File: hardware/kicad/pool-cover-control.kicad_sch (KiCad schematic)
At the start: 70 parts, among them J1 Power_Supply _Conn, J2 Motor_Conn, J3 Key_Switch_Conn, J4 Limit_Switch_Conn, J5 SWD_Conn, Q1 DMP4015SK3Q-13, U1 STM32G031K8Tx, U2 ULN2003A, U3 LMR14206, U4 PC817, U5 PC817, U6 PC817, U7 PC817

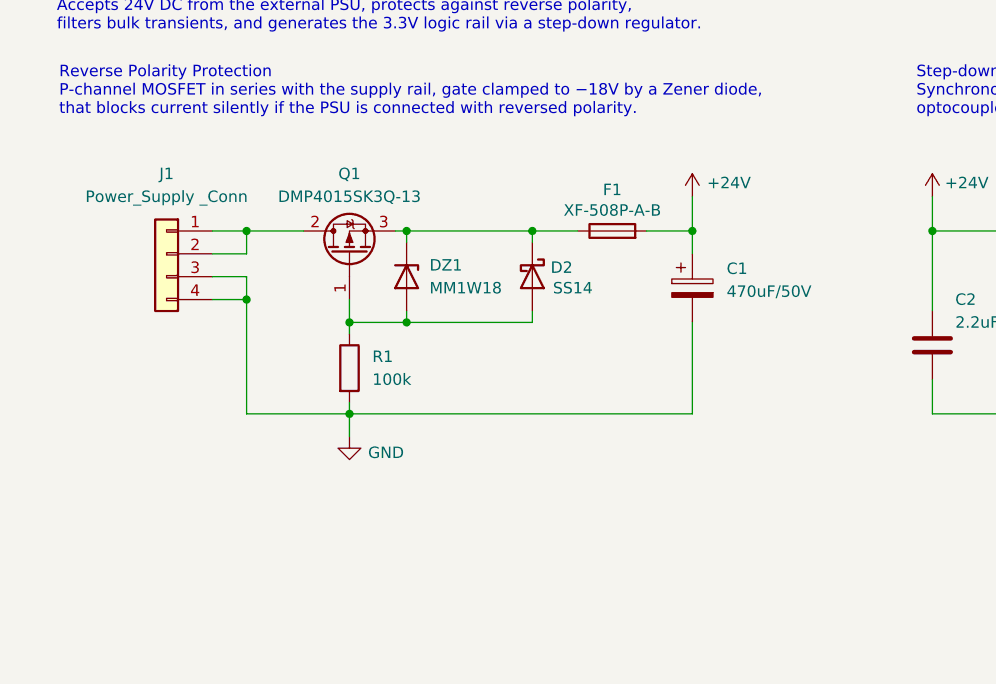
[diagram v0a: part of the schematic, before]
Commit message: feat(hardware): implement pcb layout
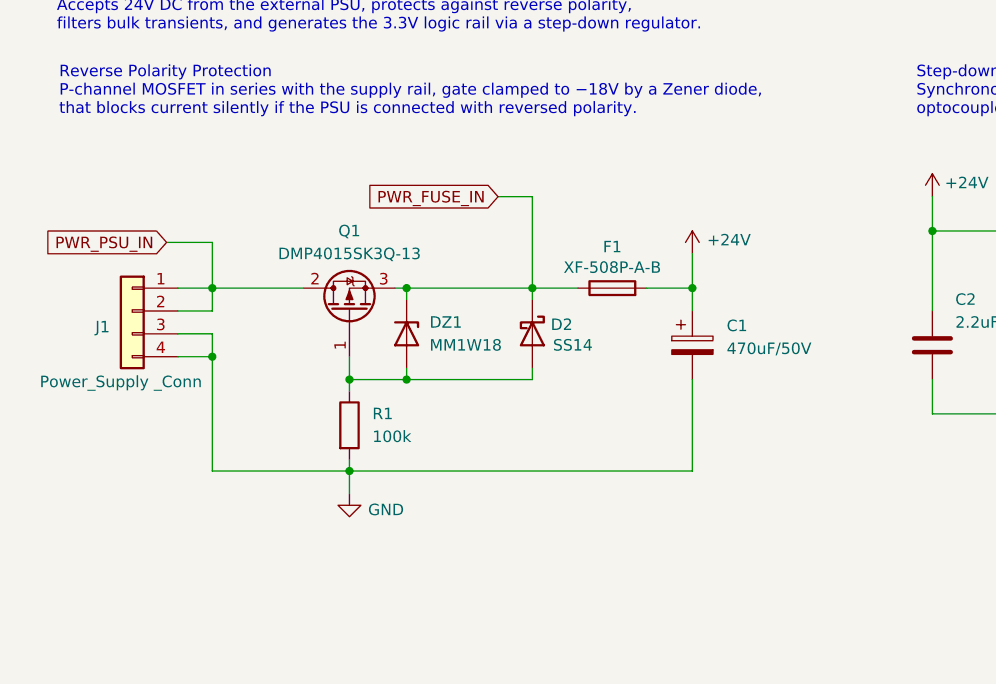
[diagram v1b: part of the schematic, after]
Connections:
- net PWR_FUSE_IN: now reaches D2.1 (K), DZ1.1 (K), F1.1, Q1.3 (S)
- net PWR_PSU_IN: now reaches J1.1 (Pin_1), J1.2 (Pin_2), Q1.2 (D)
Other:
- moved on the sheet: C1, D2, DZ1, F1, J1, Q1, R1
